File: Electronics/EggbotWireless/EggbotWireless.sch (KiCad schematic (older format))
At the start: 55 parts, among them J1 BATT, J2 Conn_01x04_Female, J3 USB_B_Micro, J4 AVR-ISP-6, J5 Conn_01x03_Female, M1 Stepper_Motor_bipolar, M2 Stepper_Motor_bipolar, Q1 FDD8447L, U1 TPS62203DBV, U2 ATmega16A-AU, U3 DW01, U4 FS8205A, U5 CP2102-GMR, U6 LTC4054ES5-4.2, U7 ESP-12E, U8 LM3478, Y1 16MHz

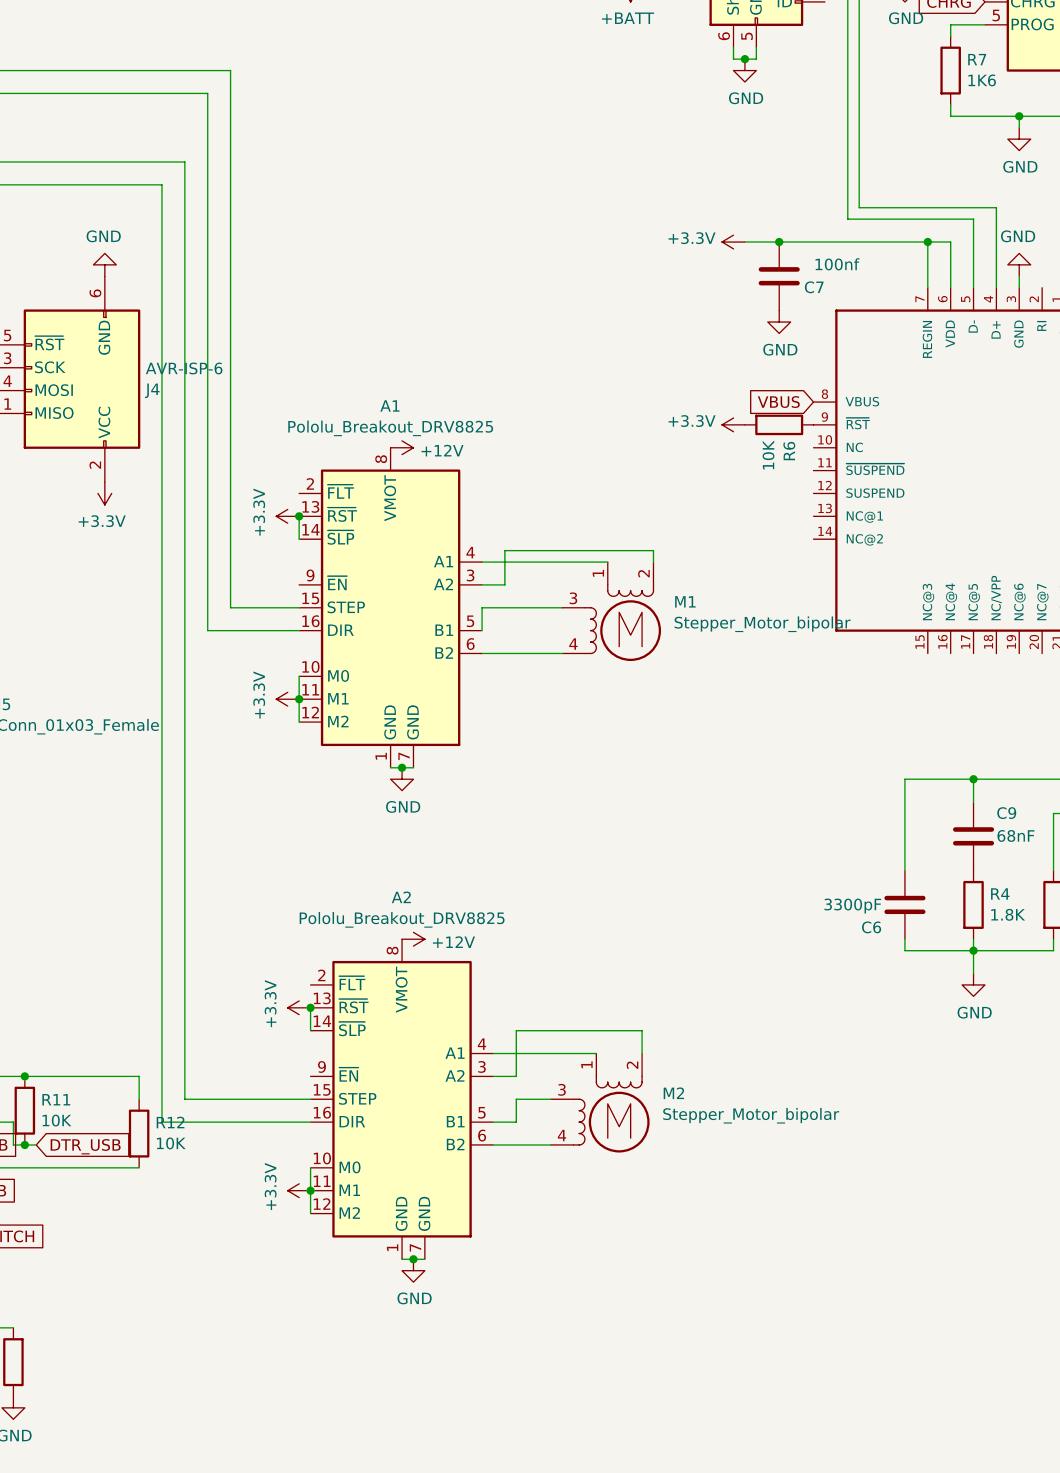
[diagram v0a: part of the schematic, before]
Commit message: add branding
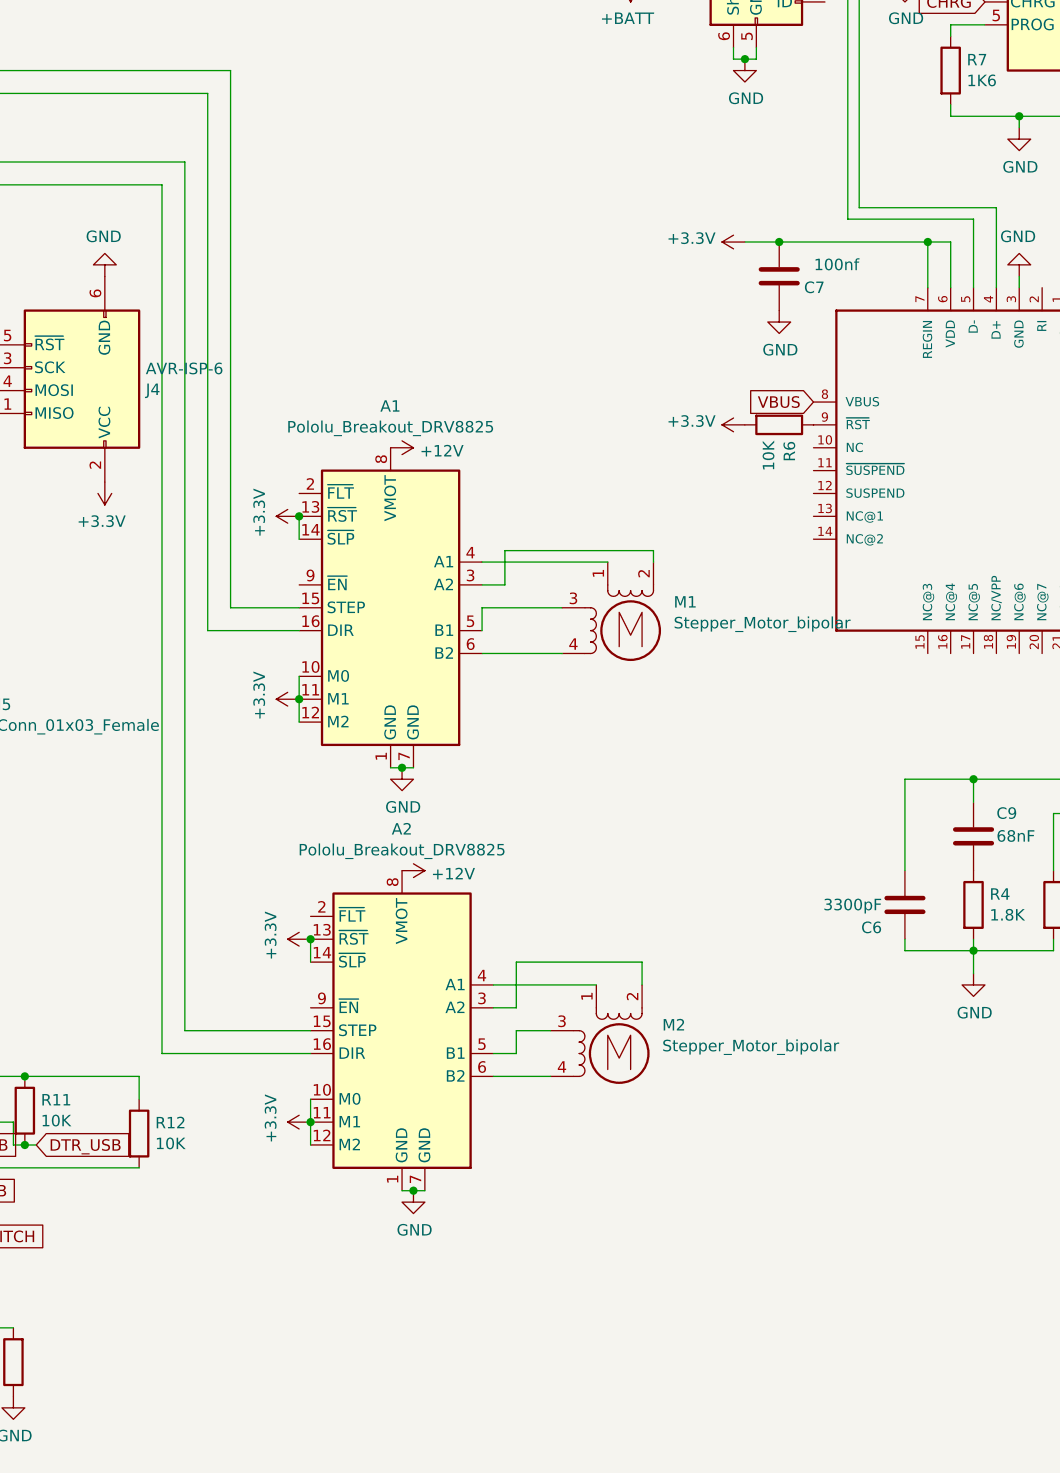
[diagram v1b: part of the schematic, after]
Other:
- moved on the sheet: A2, M2
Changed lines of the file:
@@
 L Motor:Stepper_Motor_bipolar M2
 U 1 1 5CF4C34B
-P 5950 6100
-F 0 "M2" H 6138 6224 50  0000 L CNN
-F 1 "Stepper_Motor_bipolar" H 6138 6133 50  0000 L CNN
-F 2 "Connector_PinSocket_2.54mm:PinSocket_1x04_P2.54mm_Vertical" H 5960 6090 50  0001 C CNN
-F 3 "http://www.infineon.com/dgdl/Application-Note-TLE8110EE_driving_UniPolarStepperMotor_V1.1.pdf?fileId=db3a30431be39b97011be5d0aa0a00b0" H 5960 6090 50  0001 C CNN
-	1    5950 6100
+P 5950 5800
+F 0 "M2" H 6138 5924 50  0000 L CNN
+F 1 "Stepper_Motor_bipolar" H 6138 5833 50  0000 L CNN
+F 2 "Connector_PinSocket_2.54mm:PinSocket_1x04_P2.54mm_Vertical" H 5960 5790 50  0001 C CNN
+F 3 "http://www.infineon.com/dgdl/Application-Note-TLE8110EE_driving_UniPolarStepperMotor_V1.1.pdf?fileId=db3a30431be39b97011be5d0aa0a00b0" H 5960 5790 50  0001 C CNN
+	1    5950 5800
 	1    0    0    -1
 $EndComp
@@
 L Driver_Motor:Pololu_Breakout_DRV8825 A2
 U 1 1 5CE8A6D5
-P 5000 5900
-F 0 "A2" H 5000 6681 50  0000 C CNN
-F 1 "Pololu_Breakout_DRV8825" H 5000 6590 50  0000 C CNN
-F 2 "Module:Pololu_Breakout-16_15.2x20.3mm" H 5200 5100 50  0001 L CNN
-F 3 "https://www.pololu.com/product/2982" H 5100 5600 50  0001 C CNN
-	1    5000 5900
+P 5000 5600
+F 0 "A2" H 5000 6381 50  0000 C CNN
+F 1 "Pololu_Breakout_DRV8825" H 5000 6290 50  0000 C CNN
+F 2 "Module:Pololu_Breakout-16_15.2x20.3mm" H 5200 4800 50  0001 L CNN
+F 3 "https://www.pololu.com/product/2982" H 5100 5300 50  0001 C CNN
+	1    5000 5600
 	1    0    0    -1
 $EndComp
@@
 	5700 4050 5350 4050
 Wire Wire Line
-	5850 5800 5400 5800
-Wire Wire Line
-	6050 5800 6050 5700
-Wire Wire Line
-	6050 5700 5500 5700
-Wire Wire Line
-	5500 5700 5500 5900
-Wire Wire Line
-	5500 5900 5400 5900
-Wire Wire Line
-	5650 6000 5500 6000
-Wire Wire Line
-	5500 6000 5500 6100
-Wire Wire Line
-	5500 6100 5400 6100
-Wire Wire Line
-	5650 6200 5400 6200
+	5850 5500 5400 5500
+Wire Wire Line
+	6050 5500 6050 5400
+Wire Wire Line
+	6050 5400 5500 5400
+Wire Wire Line
+	5500 5400 5500 5600
+Wire Wire Line
+	5500 5600 5400 5600
+Wire Wire Line
+	5650 5700 5500 5700
+Wire Wire Line
+	5500 5700 5500 5800
+Wire Wire Line
+	5500 5800 5400 5800
+Wire Wire Line
+	5650 5900 5400 5900
 $Comp
 L power:+12V #PWR?
 U 1 1 5CF0714E
-P 5000 5300
-F 0 "#PWR?" H 5000 5150 50  0001 C CNN
-F 1 "+12V" V 5015 5428 50  0000 L CNN
-F 2 "" H 5000 5300 50  0001 C CNN
-F 3 "" H 5000 5300 50  0001 C CNN
-	1    5000 5300
+P 5000 5000
+F 0 "#PWR?" H 5000 4850 50  0001 C CNN
+F 1 "+12V" V 5015 5128 50  0000 L CNN
+F 2 "" H 5000 5000 50  0001 C CNN
+F 3 "" H 5000 5000 50  0001 C CNN
+	1    5000 5000
 	0    1    1    0
 $EndComp
@@
 L EggbotWireless-rescue:GND-power-Catfi-rescue #PWR?
 U 1 1 5CF0A85A
-P 5050 6700
-F 0 "#PWR?" H 5050 6450 50  0001 C CNN
-F 1 "GND" H 5055 6527 50  0000 C CNN
-F 2 "" H 5050 6700 50  0001 C CNN
-F 3 "" H 5050 6700 50  0001 C CNN
-	1    5050 6700
-	1    0    0    -1
-$EndComp
-Wire Wire Line
-	5100 6700 5050 6700
-Wire Wire Line
-	5000 6700 5050 6700
-Connection ~ 5050 6700
+P 5050 6400
+F 0 "#PWR?" H 5050 6150 50  0001 C CNN
+F 1 "GND" H 5055 6227 50  0000 C CNN
+F 2 "" H 5050 6400 50  0001 C CNN
+F 3 "" H 5050 6400 50  0001 C CNN
+	1    5050 6400
+	1    0    0    -1
+$EndComp
+Wire Wire Line
+	5100 6400 5050 6400
+Wire Wire Line
+	5000 6400 5050 6400
+Connection ~ 5050 6400
 $Comp
 L EggbotWireless-rescue:GND-power-Catfi-rescue #PWR?
@@
 Connection ~ 5000 4550
 Wire Wire Line
-	4600 6300 4600 6400
-Connection ~ 4600 6400
-Wire Wire Line
-	4600 6400 4600 6500
+	4600 6000 4600 6100
+Connection ~ 4600 6100
+Wire Wire Line
+	4600 6100 4600 6200
 Wire Wire Line
 	4550 4350 4550 4250
@@
 L power:+3.3V #PWR?
 U 1 1 5CF86B51
-P 4600 6400
-F 0 "#PWR?" H 4600 6250 50  0001 C CNN
-F 1 "+3.3V" H 4615 6573 50  0000 C CNN
-F 2 "" H 4600 6400 50  0001 C CNN
-F 3 "" H 4600 6400 50  0001 C CNN
-	1    4600 6400
+P 4600 6100
+F 0 "#PWR?" H 4600 5950 50  0001 C CNN
+F 1 "+3.3V" H 4615 6273 50  0000 C CNN
+F 2 "" H 4600 6100 50  0001 C CNN
+F 3 "" H 4600 6100 50  0001 C CNN
+	1    4600 6100
 	0    -1   -1   0
 $EndComp
@@
 L power:+3.3V #PWR?
 U 1 1 5CF94114
-P 4600 5600
-F 0 "#PWR?" H 4600 5450 50  0001 C CNN
-F 1 "+3.3V" H 4615 5773 50  0000 C CNN
-F 2 "" H 4600 5600 50  0001 C CNN
-F 3 "" H 4600 5600 50  0001 C CNN
-	1    4600 5600
-	0    -1   -1   0
-$EndComp
-Wire Wire Line
-	4600 5600 4600 5700
-Connection ~ 4600 5600
+P 4600 5300
+F 0 "#PWR?" H 4600 5150 50  0001 C CNN
+F 1 "+3.3V" H 4615 5473 50  0000 C CNN
+F 2 "" H 4600 5300 50  0001 C CNN
+F 3 "" H 4600 5300 50  0001 C CNN
+	1    4600 5300
+	0    -1   -1   0
+$EndComp
+Wire Wire Line
+	4600 5300 4600 5400
+Connection ~ 4600 5300
 $Comp
 L power:+3.3V #PWR?
@@
 	4150 1600 2750 1600
 Wire Wire Line
-	4600 6000 4050 6000
-Wire Wire Line
-	4050 6000 4050 1900
+	4600 5700 4050 5700
 Wire Wire Line
 	4050 1900 2750 1900
 Wire Wire Line
-	4600 6100 3950 6100
-Wire Wire Line
-	3950 6100 3950 2000
+	4600 5800 3950 5800
 Wire Wire Line
 	3950 2000 2750 2000
+Wire Wire Line
+	4050 1900 4050 5700
+Wire Wire Line
+	3950 2000 3950 5800
 $EndSCHEMATC
